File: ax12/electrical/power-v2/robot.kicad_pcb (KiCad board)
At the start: 2 copper layers, 49.5 x 49.5 mm, 33 parts, among them J1 LEG1, J2 LEG2, J3 LEG4, J4 LEG3, J5 Data P, J6 PWR IN, U1 LM317_12, U2 LM317_12, U3 LM317_34, U4 LM317_34

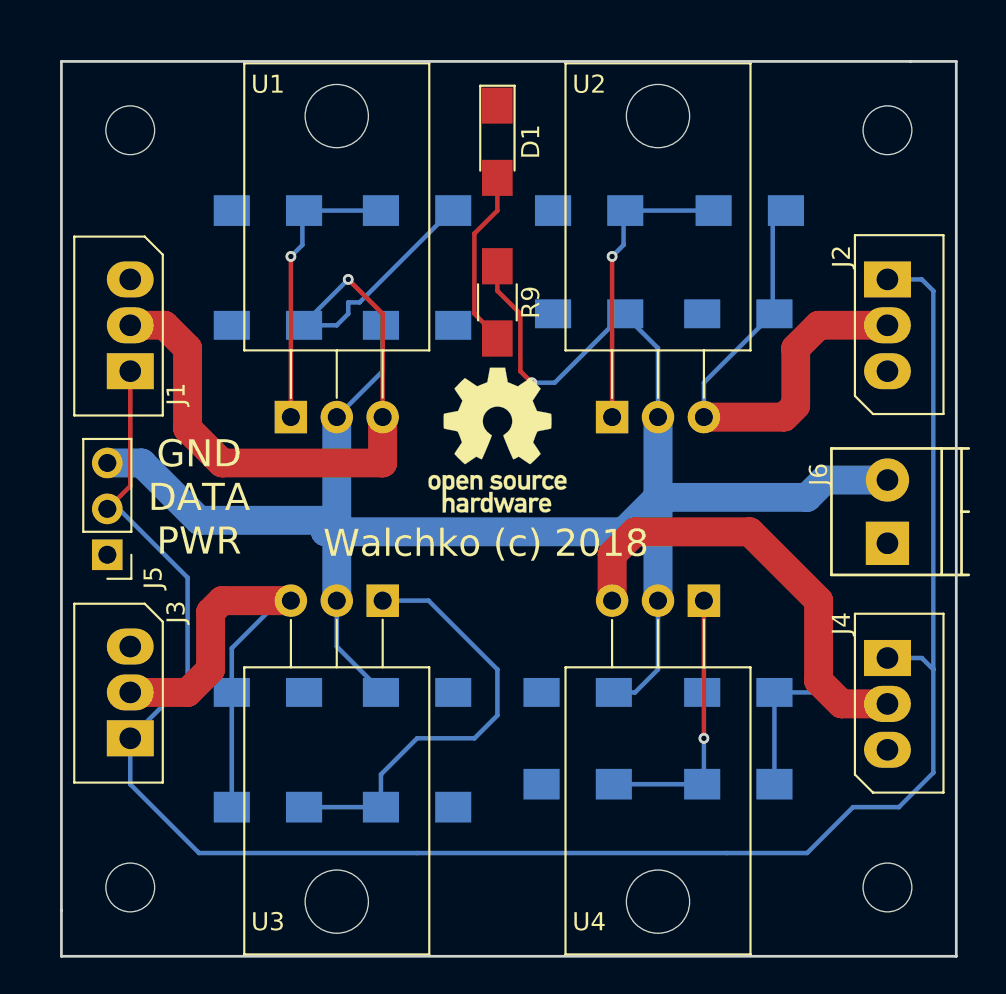
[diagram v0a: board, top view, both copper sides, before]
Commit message: new power board
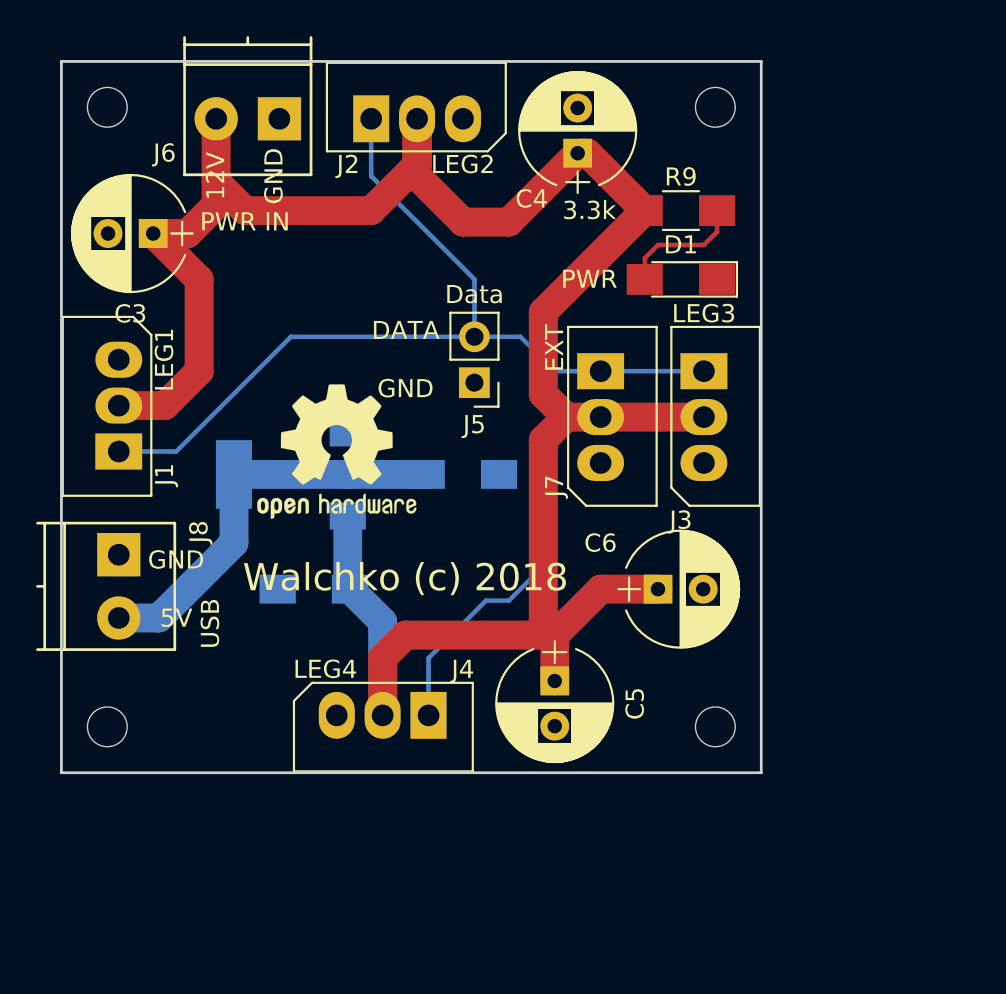
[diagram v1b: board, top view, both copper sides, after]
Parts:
- removed the ? at (154.9, 63.5)
- removed the ? at (113.0, 63.5)
- removed the ? at (113.0, 105.4)
- removed the ? at (154.9, 105.4)
- removed the ? at (133.3, 80.6)
- removed C7, C8: C, Capacitors_SMD:C_1206_HandSoldering
- removed R1, R3, R5, R7: 390, Resistors_SMD:R_1206_HandSoldering
- removed R2, R4, R6, R8: 3.3k, Resistors_SMD:R_1206_HandSoldering
- removed U2: LM317_12, TO_SOT_Packages_THT:TO-220-3_Horizontal
- removed U3, U4: LM317_34, TO_SOT_Packages_THT:TO-220-3_Horizontal
- added ?: MountingHole_2.2mm_M2, Mounting_Holes:MountingHole_2.2mm_M2, F.Cu at (145.4, 62.2)
- added ?: MountingHole_2.2mm_M2, Mounting_Holes:MountingHole_2.2mm_M2, F.Cu at (111.8, 62.2)
- added ?: , Mounting_Holes:MountingHole_2.2mm_M2, F.Cu at (111.8, 96.5)
- added ?: , Mounting_Holes:MountingHole_2.2mm_M2, F.Cu at (145.4, 96.5)
- added J7: EXT, Connectors_Molex:Molex_SPOX-5267_22-03-5035_03x2.54mm_Straight, F.Cu at (139.1, 76.8)
- added J8: USB, TerminalBlocks_Phoenix:TerminalBlock_Phoenix_PT-3.5mm_2pol, F.Cu at (112.4, 87.0)
- added REF***: OSHW-Logo2_9.8x8mm_SilkScreen, Symbols:OSHW-Logo2_9.8x8mm_SilkScreen, F.Cu at (124.5, 81.3)
- added REF***: KiCad-Logo2_12mm_SilkScreen, Symbols:KiCad-Logo2_12mm_SilkScreen, B.Cu at (129.5, 70.5)
- C3, C4, C5, C6: footprint Capacitors_SMD:C_1206_HandSoldering -> Capacitors_THT:CP_Radial_D6.3mm_P2.50mm; moved to F.Cu
- J3: value LEG4 -> LEG3
- J4: value LEG3 -> LEG4
- J5: value Data P -> Data; footprint Pin_Headers:Pin_Header_Straight_1x03_Pitch2.54mm -> Pin_Headers:Pin_Header_Straight_1x02_Pitch2.54mm
- R9: value 330 -> 3.3k
- U1: value LM317_12 -> AP1117-50; footprint TO_SOT_Packages_THT:TO-220-3_Horizontal -> ksmd:SOT-223-3_TabPin2; moved to B.Cu
- moved J6 41.0 mm to (121.3, 62.9), turned to 180 degrees
- moved J3 37.7 mm to (144.8, 76.8), turned to 270 degrees
- moved J2 29.9 mm to (126.4, 62.9), turned to 0 degrees
- moved J4 25.6 mm to (129.5, 95.9), turned to 180 degrees
- moved J5 22.4 mm to (132.1, 77.5)
- moved C2 21.6 mm to (123.2, 88.9)
- moved C5 15.9 mm to (136.5, 94.0), turned to 270 degrees
- moved D1 12.7 mm to (143.5, 71.8), turned to 180 degrees
- moved C4 12.6 mm to (137.8, 64.8), turned to 90 degrees
- moved R9 11.4 mm to (143.5, 67.9), turned to 0 degrees
- moved C1 8.64 mm to (131.4, 82.5)
- moved C3 8.13 mm to (114.3, 69.2)
- moved C6 7.24 mm to (142.2, 88.9), turned to 0 degrees
- moved J1 4.49 mm to (112.4, 81.3)
- moved U1 3.17 mm to (121.9, 82.5), turned to 180 degrees
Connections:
- C1 pad 1: +VDC -> +5V
- C1 pad 2: GNDA -> GND
- C2 pad 1: +VDC -> +12V
- C2 pad 2: GNDA -> GND
- C3 pad 1: Net-(C3-Pad1) -> +12V
- C3 pad 2: GNDA -> GND
- C4 pad 1: Net-(C4-Pad1) -> +12V
- C4 pad 2: GNDA -> GND
- C5 pad 1: Net-(C5-Pad1) -> +12V
- C5 pad 2: GNDA -> GND
- C6 pad 1: Net-(C6-Pad1) -> +12V
- C6 pad 2: GNDA -> GND
- D1 pad 1: GNDA -> GND
- J1 pad 2: Net-(C3-Pad1) -> +12V
- J1 pad 3: GNDA -> GND
- J2 pad 2: Net-(C4-Pad1) -> +12V
- J2 pad 3: GNDA -> GND
- J3 pad 2: Net-(C5-Pad1) -> +12V
- J3 pad 3: GNDA -> GND
- J4 pad 2: Net-(C6-Pad1) -> +12V
- J4 pad 3: GNDA -> GND
- J5 pad 1: GNDA -> GND
- J6 pad 1: GNDA -> GND
- J6 pad 2: +VDC -> +12V
- R9 pad 1: +VDC -> +12V
- U1 pad 1: Net-(R1-Pad2) -> GND
- U1 pad 2: +VDC -> +5V
- U1 pad 3: Net-(C3-Pad1) -> +12V
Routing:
- net +12V: track 0.00 -> 126.8 mm
- net +VDC: track 107.2 -> 0.00 mm, vias 1 -> 0
- net Net-(C3-Pad1): track 45.6 -> 0.00 mm, vias 1 -> 0
- net Net-(C6-Pad1): track 36.5 -> 0.00 mm
- net DATA: track 107.1 -> 72.9 mm
- net Net-(C4-Pad1): track 27.7 -> 0.00 mm
- net Net-(C5-Pad1): track 26.0 -> 0.00 mm
- net Net-(R5-Pad2): track 24.3 -> 0.00 mm
- net +5V: track 0.00 -> 22.6 mm
- net Net-(R3-Pad2): track 16.7 -> 0.00 mm, vias 1 -> 0
- net Net-(R1-Pad2): track 16.0 -> 0.00 mm, vias 1 -> 0
- net Net-(R7-Pad2): track 15.1 -> 0.00 mm, vias 1 -> 0
- net Net-(D1-Pad2): track 9.94 -> 6.95 mm
- added copper zone on B.Cu, net GND
- added copper zone on F.Cu, net GND
- removed copper zone on B.Cu, net GNDA
- removed copper zone on F.Cu, net GNDA
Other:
- board size 49.5 x 49.5 mm -> 38.7 x 39.4 mm
- net class high added: clearance 0.3, trace_width 2.1, via_dia 0.6, via_drill 0.4
- net class large removed
- board text added: "12V GND"
- board text added: "DATA GND"
- board text added: "GND 5V"
- board text removed: "GND DATA PWR"
